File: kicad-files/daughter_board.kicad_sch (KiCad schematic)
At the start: 14 parts, among them J1 TYPE-C-31-M12_13, T1 53261-0471, U2 USBLC6-2SC6, U4 SGM2007-3.3XN5/TR

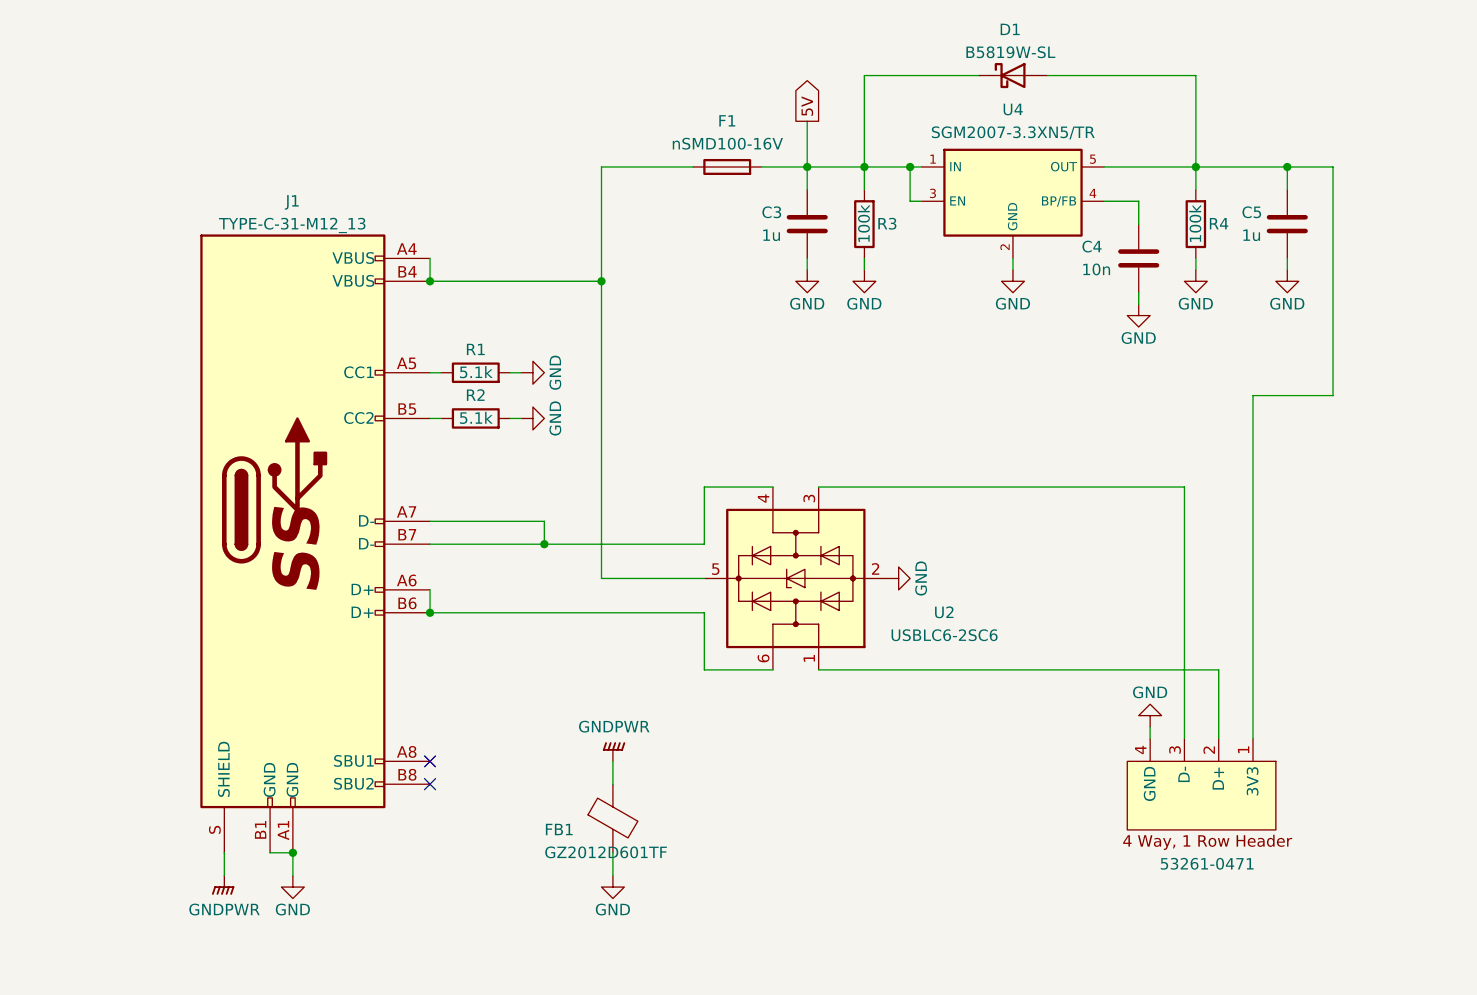
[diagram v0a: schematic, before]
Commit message: Fixed up the daughter board
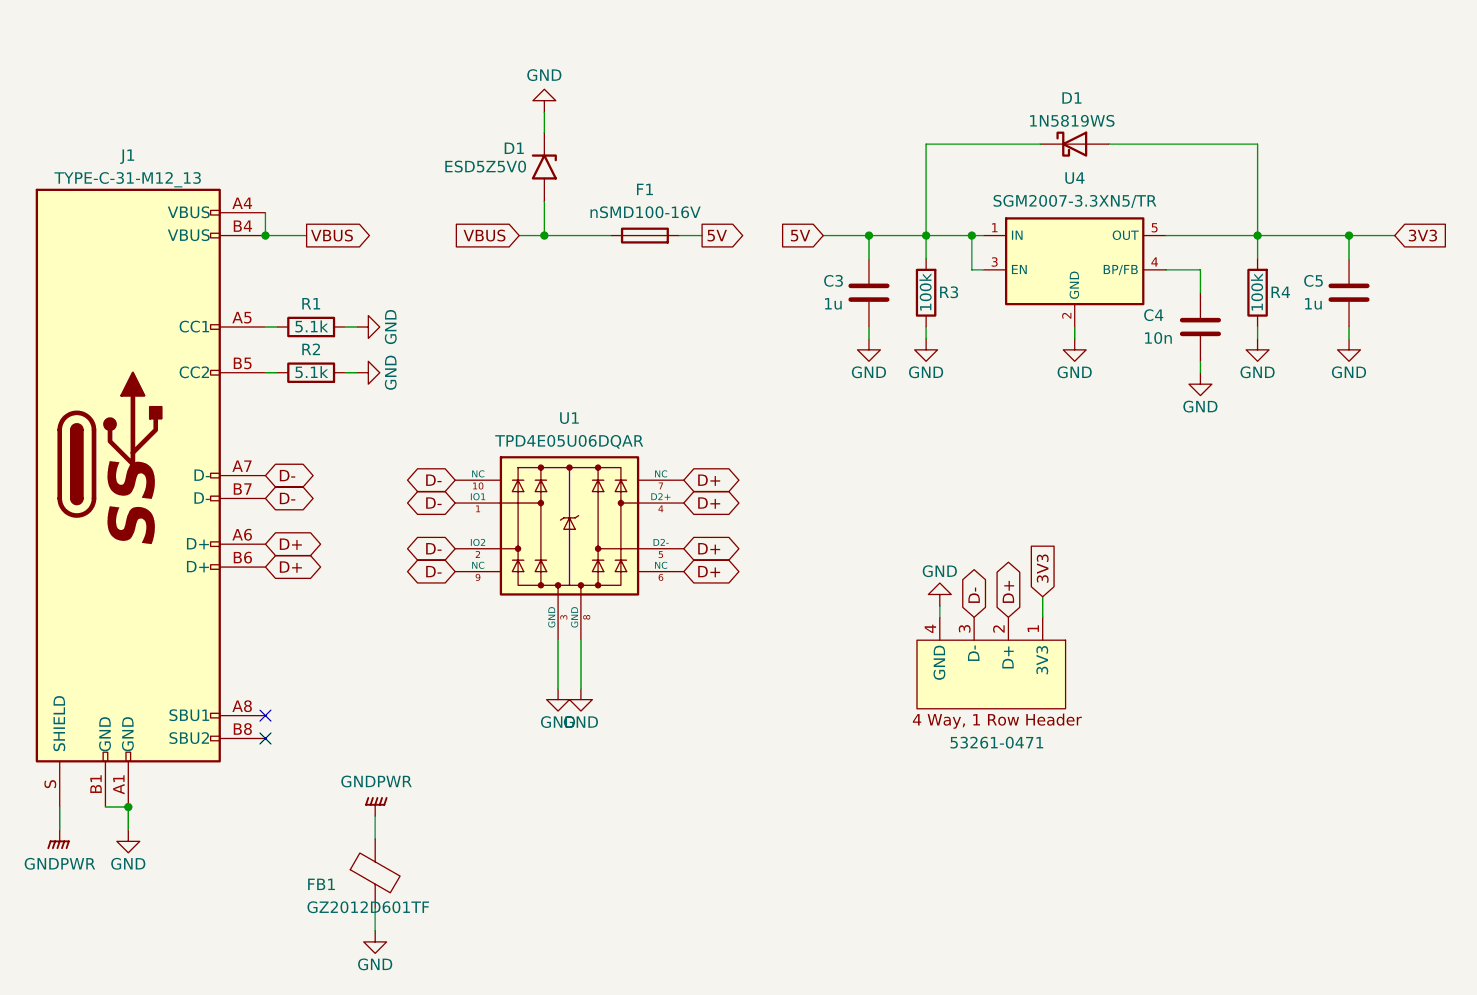
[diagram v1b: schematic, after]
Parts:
- removed U2: USBLC6-2SC6, acheron_Components:SOT-23-6, symbol Power_Protection:USBLC6-2SC6
- added D1: ESD5Z5V0, Diode_SMD:D_SOD-523, symbol Diode:SMF6V0A
- added U1: TPD4E05U06DQAR, Package_SON:USON-10_2.5x1.0mm_P0.5mm, symbol acheron_Symbols:TPD4E05U06DQAR
- D1: value B5819W-SL -> 1N5819WS; footprint Diode_SMD:D_SOD-123 -> Diode_SMD:D_SOD-323
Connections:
- net GND: now also D1.1 (A1), U1.3 (GND), U1.8 (GND)
- net 3V3: now reaches C5.1, D1.2 (A), R4.2, T1.1 (3V3), U4.5 (OUT)
- net VBUS: now reaches F1.1, J1.A4 (VBUS), J1.B4 (VBUS)
- net VBUS: now also D1.2 (A2)
- net D+: now reaches T1.2 (D+)
- net D+: now also J1.A6 (D+), J1.B6 (D+), U1.4 (D2+), U1.5 (D2-), U1.6 (NC), U1.7 (NC)
- net D-: now reaches T1.3 (D-)
- net D-: now also J1.A7 (D-), J1.B7 (D-), U1.1 (IO1), U1.10 (NC), U1.2 (IO2), U1.9 (NC)
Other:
- moved on the sheet: C3, C4, C5, D1, F1, FB1, J1, R1, R2, R3, R4, U4
